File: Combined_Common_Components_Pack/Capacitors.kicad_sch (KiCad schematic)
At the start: 19 parts

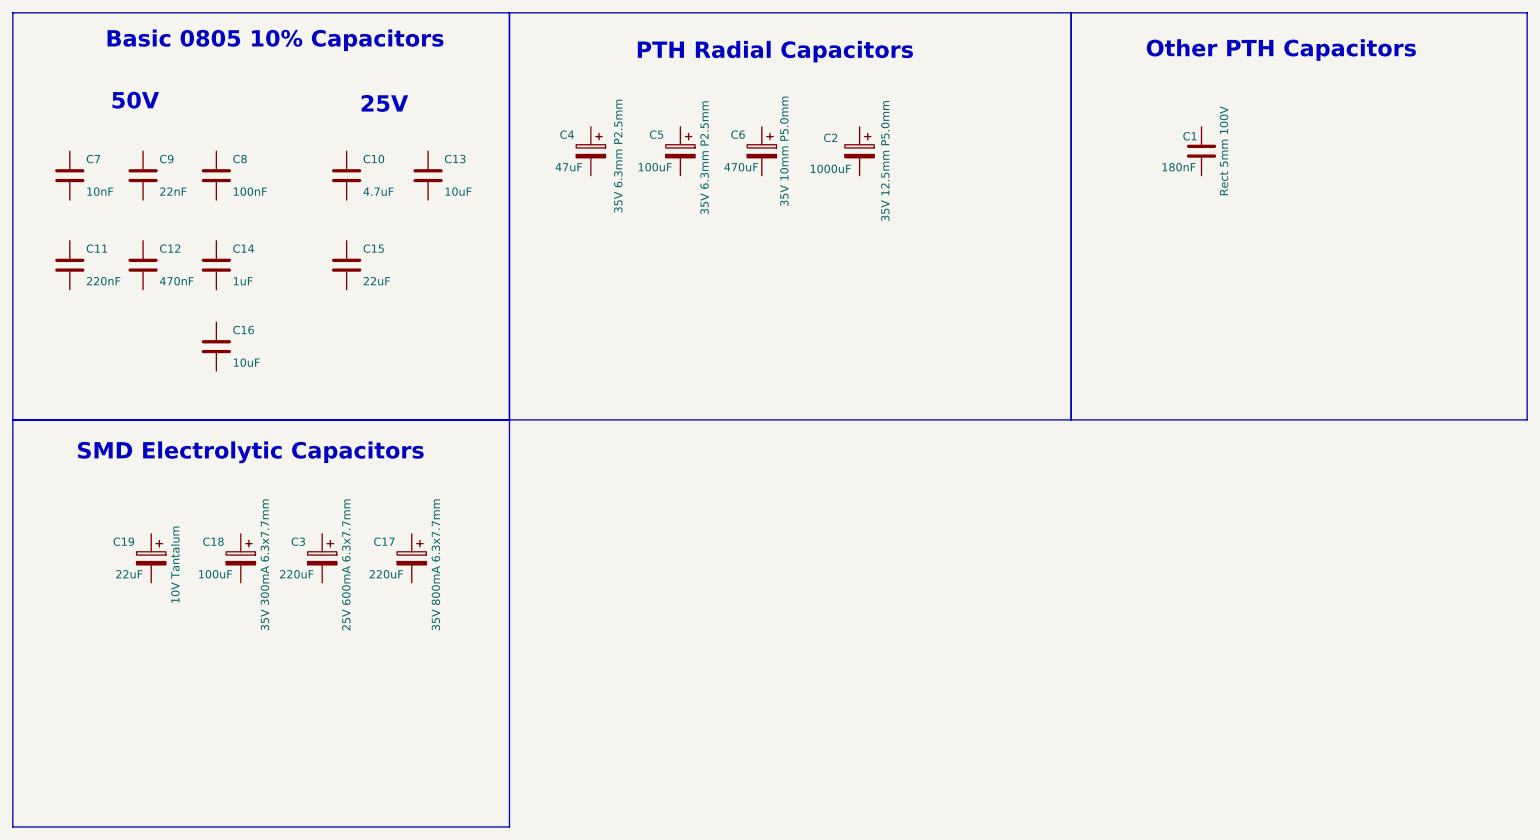
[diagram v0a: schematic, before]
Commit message: Added some connectors and basic parts
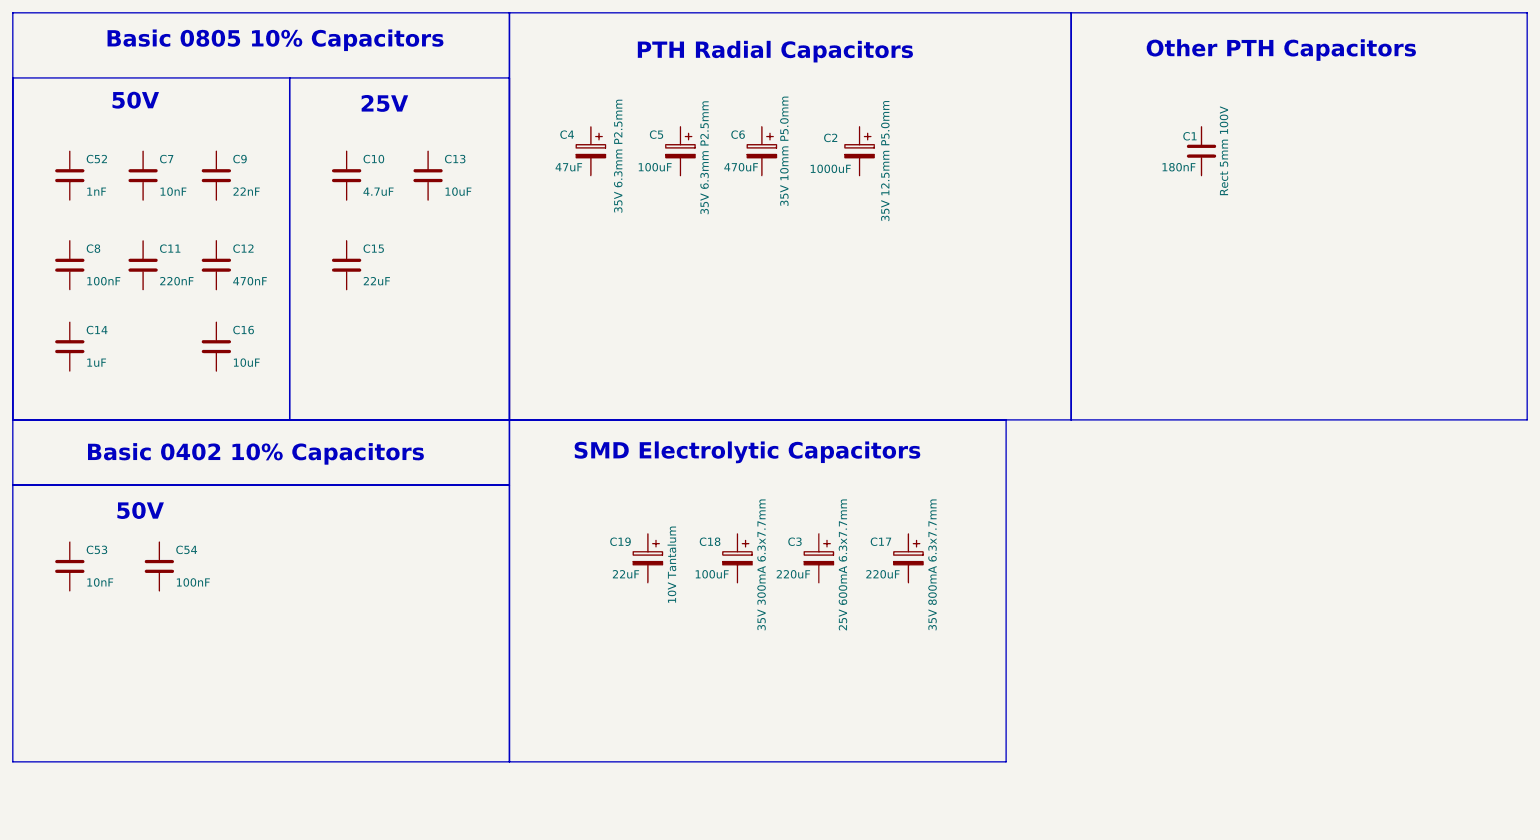
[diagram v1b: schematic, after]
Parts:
- added C52: 1nF, Capacitor_SMD:C_0805_2012Metric, symbol Device:C
- added C53: 10nF, Capacitor_SMD:C_0805_2012Metric, symbol Device:C
- added C54: 100nF, Capacitor_SMD:C_0805_2012Metric, symbol Device:C
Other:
- note added: "Basic 0402 10% Capacitors"
- moved on the sheet: C11, C12, C14, C17, C18, C19, C3, C7, C8, C9
